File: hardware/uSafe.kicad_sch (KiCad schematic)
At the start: 1 part

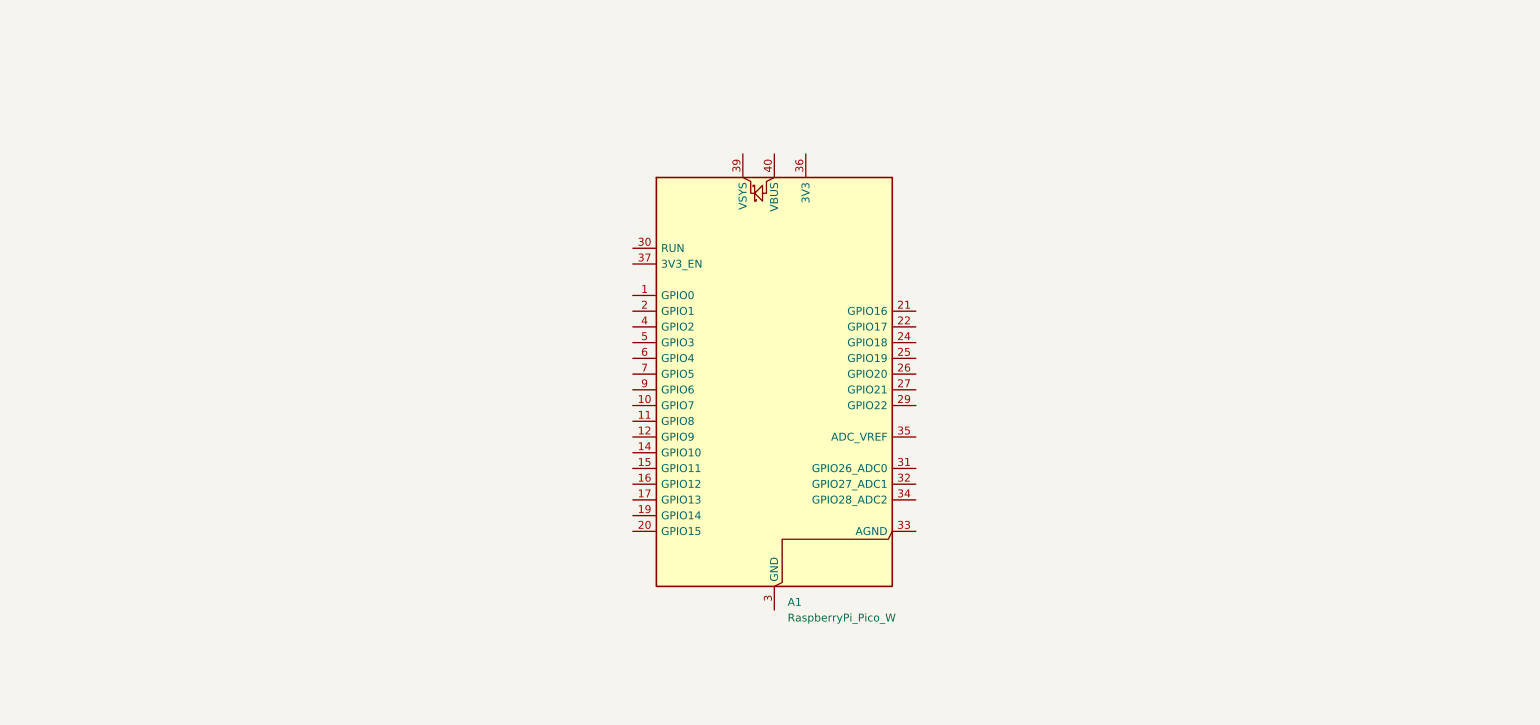
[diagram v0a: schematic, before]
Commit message: set up hardware
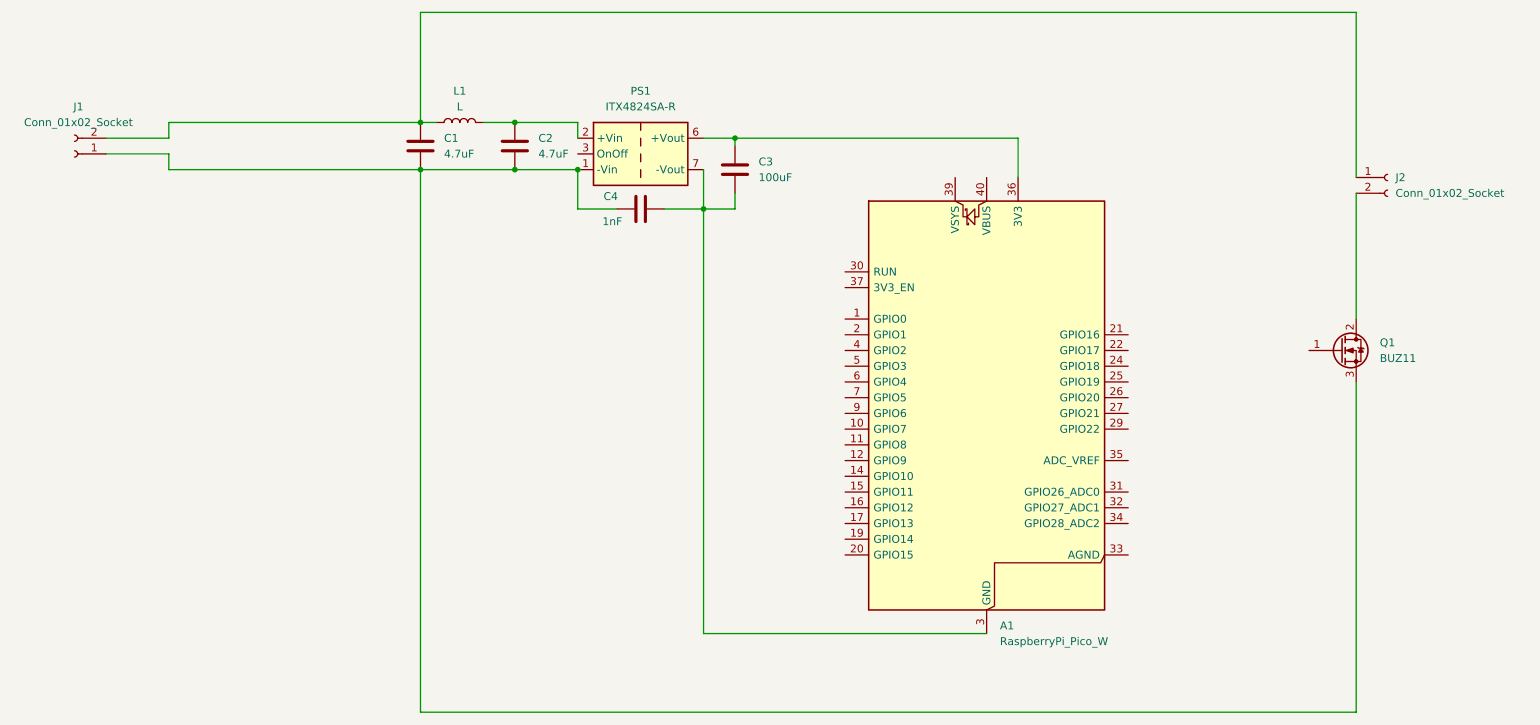
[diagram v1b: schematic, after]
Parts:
- added C1, C2: 4.7uF, symbol Device:C
- added C3: 100uF, symbol Device:C
- added C4: 1nF, symbol Device:C
- added J1, J2: Conn_01x02_Socket, symbol Connector:Conn_01x02_Socket
- added L1: L, symbol Device:L
- added PS1: ITX4824SA-R, Converter_DCDC:Converter_DCDC_XP_POWER-ITxxxxxS_THT, symbol Converter_DCDC:ITX4824SA-R
- added Q1: BUZ11, Package_TO_SOT_THT:TO-220-3_Vertical, symbol Transistor_FET:BUZ11
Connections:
- net at A1.13 (GND), A1.18 (GND), A1.23 (GND)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: now also C3.2, C4.2, PS1.7 (-Vout)
- net at A1.36 (3V3): now also C3.1, PS1.6 (+Vout)
- new net: C1.1, J1.2 (Pin_2), J2.1 (Pin_1), L1.1
- new net: C2.1, L1.2, PS1.2 (+Vin)
- new net: C1.2, C2.2, C4.1, J1.1 (Pin_1), PS1.1 (-Vin), Q1.3 (S)
- new net: J2.2 (Pin_2), Q1.2 (D)
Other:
- moved on the sheet: A1
